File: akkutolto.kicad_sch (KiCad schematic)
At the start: 12 parts, among them U1 LM317L_SOT-89, U2 LM317L_SOT-89

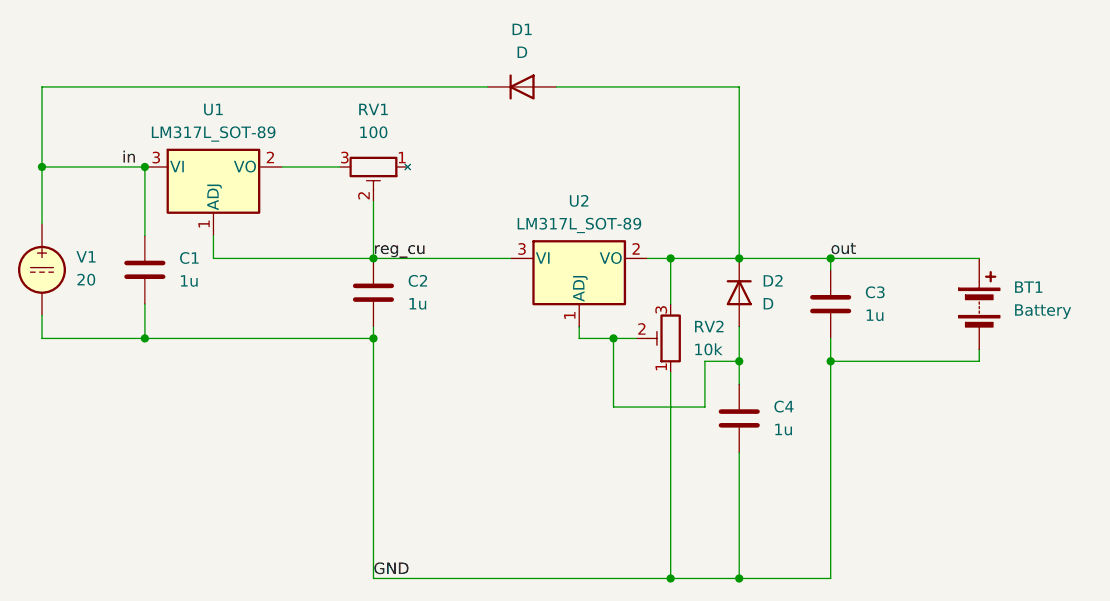
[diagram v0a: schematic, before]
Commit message: huzzad Pali
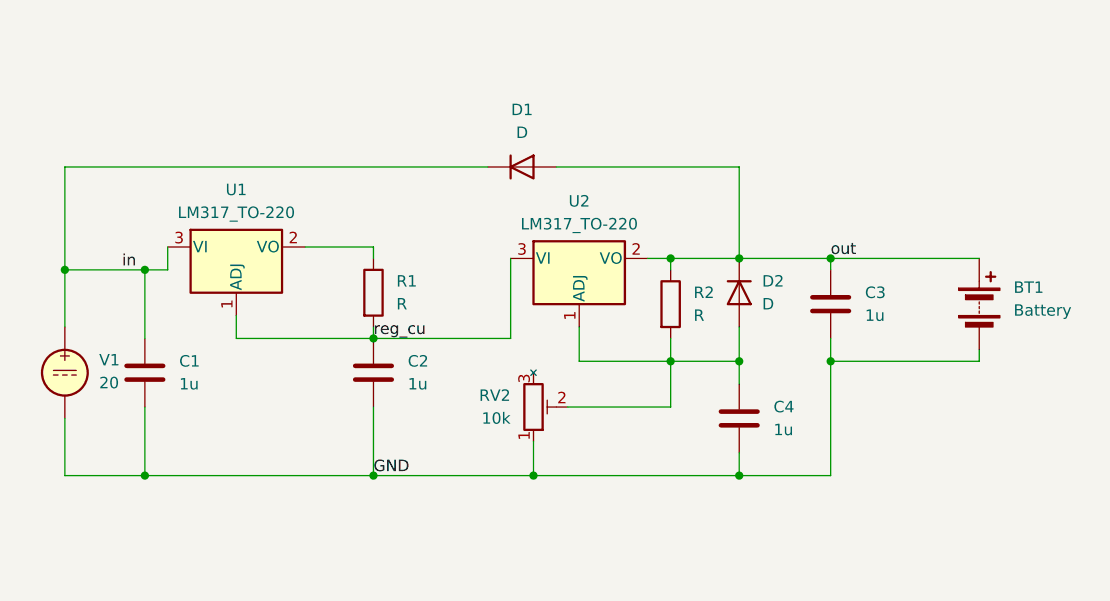
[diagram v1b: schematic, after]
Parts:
- removed RV1: 100, Potentiometer_THT:Potentiometer_Runtron_RM-065_Vertical, symbol Device:R_Potentiometer_Trim
- removed U1, U2: LM317L_SOT-89, Package_TO_SOT_SMD:SOT-89-3, symbol Regulator_Linear:LM317L_SOT-89
- added R1: R, Resistor_THT:R_Axial_Power_L25.0mm_W9.0mm_P27.94mm, symbol Device:R
- added R2: R, Resistor_SMD:R_0805_2012Metric_Pad1.20x1.40mm_HandSolder, symbol Device:R
- added U1, U2: LM317_TO-220, Package_TO_SOT_THT:TO-220-3_Horizontal_TabDown, symbol Regulator_Linear:LM317_TO-220
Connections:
- net in: now also U1.3 (VI)
- net out: now also R2.1, U2.2 (VO); no longer RV2.3
- net reg_cu: now also R1.2, U1.1 (ADJ), U2.3 (VI)
- net at C4.1, D2.2 (A), RV2.2: now also R2.2, U2.1 (ADJ)
- new net: R1.1, U1.2 (VO)
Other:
- moved on the sheet: C1, C2, D1, V1
